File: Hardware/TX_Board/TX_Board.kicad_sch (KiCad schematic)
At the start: 48 parts, among them IC1 GP2Y1+, IC2 GP2Y1+, IC3 GP2Y1+, IC4 LT3041ADE#PBF, IC5 LT3099ADE#PBF, IC6 ADPL40502AUJZ-1.5-R7, J1 Conn_Coaxial, J10 MM8030-2610RJ3, J11 MM8030-2610RJ3, J12 MM8030-2610RJ3, J2 Conn_01x01_Pin, J3 Conn_01x01_Pin, J4 Conn_01x01_Pin, J5 Conn_01x01_Pin, J6 Conn_02x12_Odd_Even, J7 Conn_01x03_Socket, J8 Conn_02x08_Odd_Even, J9 MM8030-2610RJ3, U1 SN74HCT138NSR

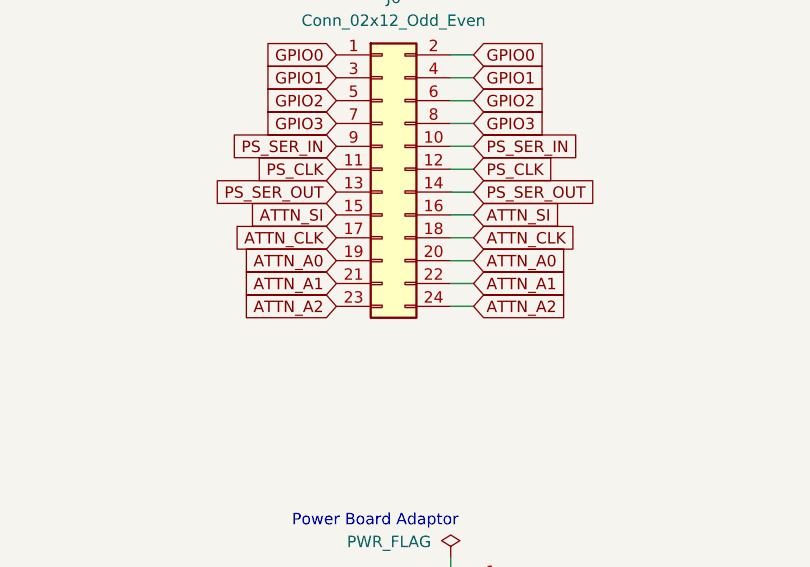
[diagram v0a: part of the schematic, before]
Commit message: DRC and more layout
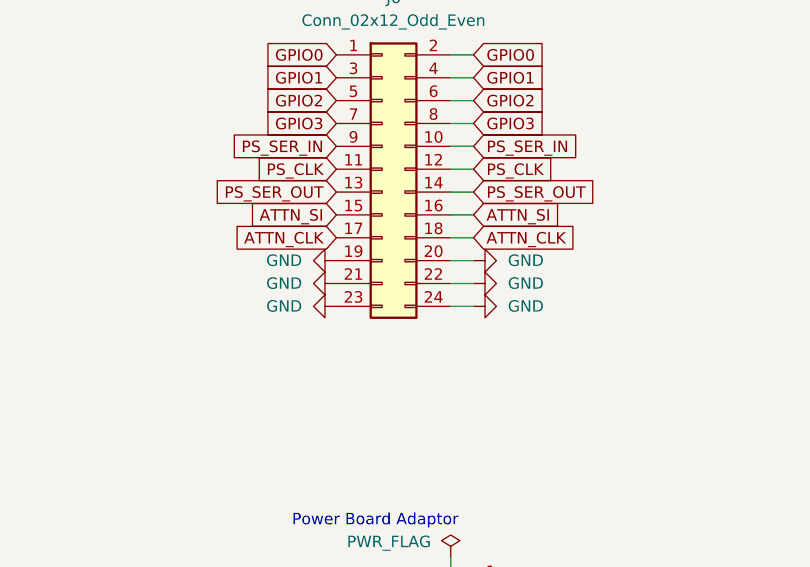
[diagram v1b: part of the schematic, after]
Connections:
- net ATTN_A0: no longer J6.19 (Pin_19), J6.20 (Pin_20)
- net ATTN_A1: no longer J6.21 (Pin_21), J6.22 (Pin_22)
- net ATTN_A2: no longer J6.23 (Pin_23), J6.24 (Pin_24)
- net GND: now also J6.19 (Pin_19), J6.20 (Pin_20), J6.21 (Pin_21), J6.22 (Pin_22), J6.23 (Pin_23), J6.24 (Pin_24)

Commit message: Gerbers
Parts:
- R4: footprint Resistor_SMD:R_0201_0603Metric -> Resistor_SMD:R_0603_1608Metric
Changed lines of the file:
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@@
 			)
 		)
-		(property "Footprint" "Resistor_SMD:R_0201_0603Metric"
+		(property "Footprint" "Resistor_SMD:R_0603_1608Metric"
 			(at 122.174 346.964 90)
 			(effects

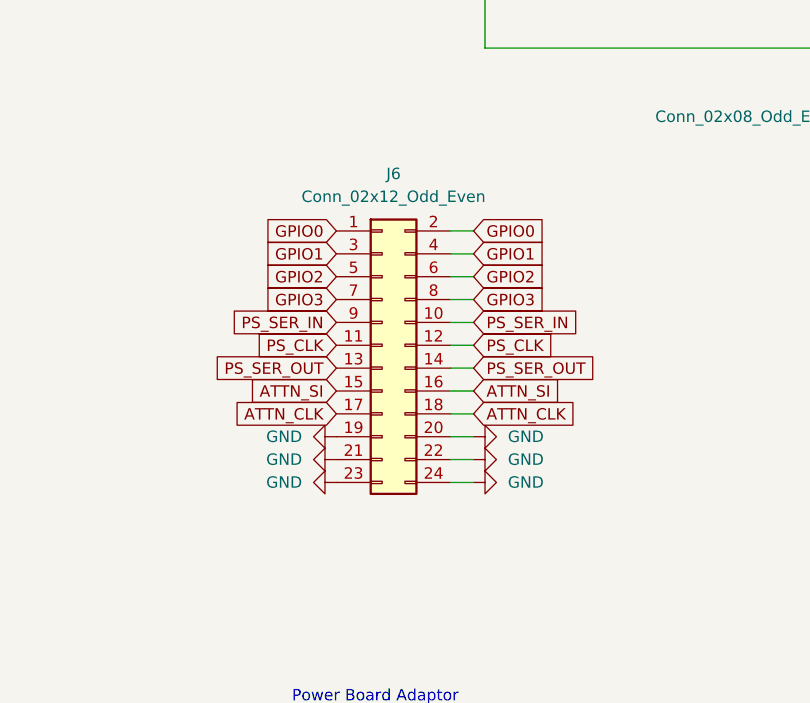
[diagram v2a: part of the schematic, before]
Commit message: Testing Data
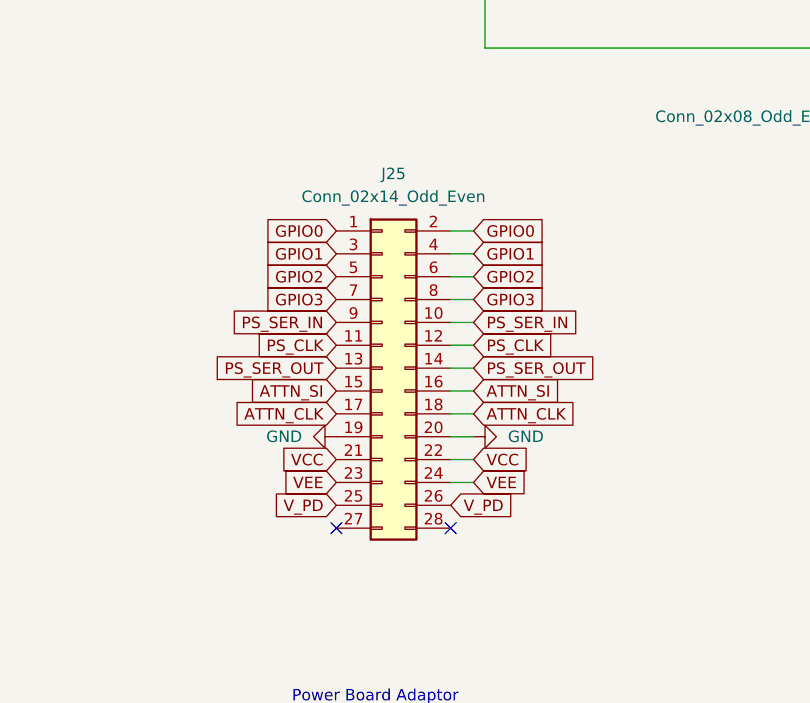
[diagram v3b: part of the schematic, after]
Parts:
- removed J6: Conn_02x12_Odd_Even, Connector_PinHeader_2.54mm:PinHeader_2x12_P2.54mm_Vertical, symbol tx_board_symbol_library:Conn_02x12_Odd_Even
- added J25: Conn_02x14_Odd_Even, Connector_PinHeader_2.54mm:PinHeader_2x14_P2.54mm_Horizontal, symbol Connector_Generic:Conn_02x14_Odd_Even
- J1: footprint Connector_Coaxial:SMA_Amphenol_132289_EdgeMount -> Connector_Coaxial:SMA_Samtec_SMA-J-P-H-ST-EM1_EdgeMount
- J8: footprint Connector_PinHeader_2.54mm:PinHeader_2x08_P2.54mm_Vertical -> Connector_PinHeader_2.54mm:PinHeader_2x08_P2.54mm_Horizontal
- R12, R13, R14, R15, R16, R17: footprint Resistor_SMD:R_0201_0603Metric -> Resistor_SMD:R_0603_1608Metric
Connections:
- net ATTN_CLK: now also J25.17 (Pin_17), J25.18 (Pin_18)
- net ATTN_SI: now also J25.15 (Pin_15), J25.16 (Pin_16)
- net GND: now also J25.19 (Pin_19), J25.20 (Pin_20)
- net GPIO0: now also J25.1 (Pin_1), J25.2 (Pin_2)
- net GPIO1: now also J25.3 (Pin_3), J25.4 (Pin_4)
- net GPIO2: now also J25.5 (Pin_5), J25.6 (Pin_6)
- net GPIO3: now also J25.7 (Pin_7), J25.8 (Pin_8)
- net PS_CLK: now also J25.11 (Pin_11), J25.12 (Pin_12)
- net PS_SER_IN: now also J25.10 (Pin_10), J25.9 (Pin_9)
- net PS_SER_OUT: now also J25.13 (Pin_13), J25.14 (Pin_14)
- net VCC: now also J25.21 (Pin_21), J25.22 (Pin_22)
- net VEE: now also J25.23 (Pin_23), J25.24 (Pin_24)
- net V_PD: now also J25.25 (Pin_25), J25.26 (Pin_26)
- no-connect marks 7 -> 9
